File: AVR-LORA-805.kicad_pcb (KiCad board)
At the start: 2 copper layers, 51.7 x 29.2 mm, 39 parts, among them J1 Batt, J2 Solar, J3 SMA, J4 CONN_01X14, J5 CONN_01X14, U1 MCP1700-3302E_SOT23, U2 RFM95HW, U3 AVR128DB28, Y1 24MHz, Y2 32768Hz

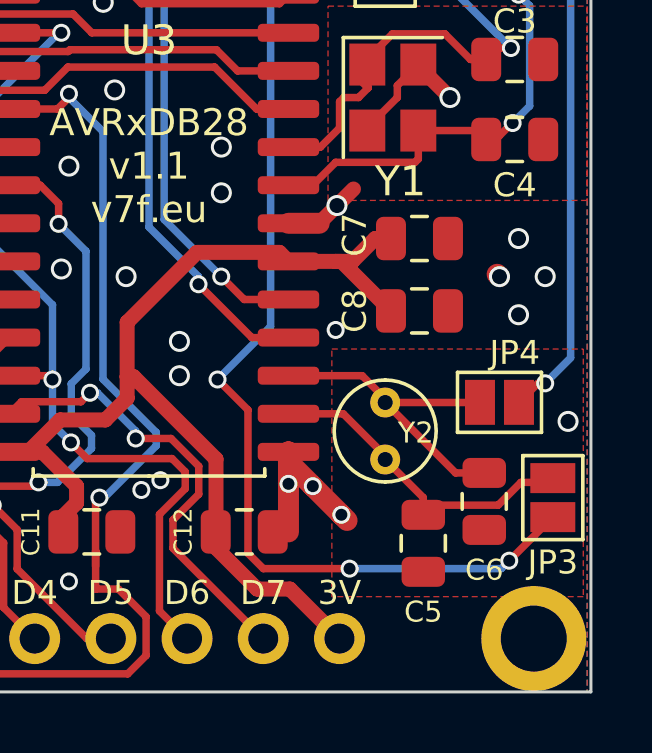
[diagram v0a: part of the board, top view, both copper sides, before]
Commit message: crystal grounding
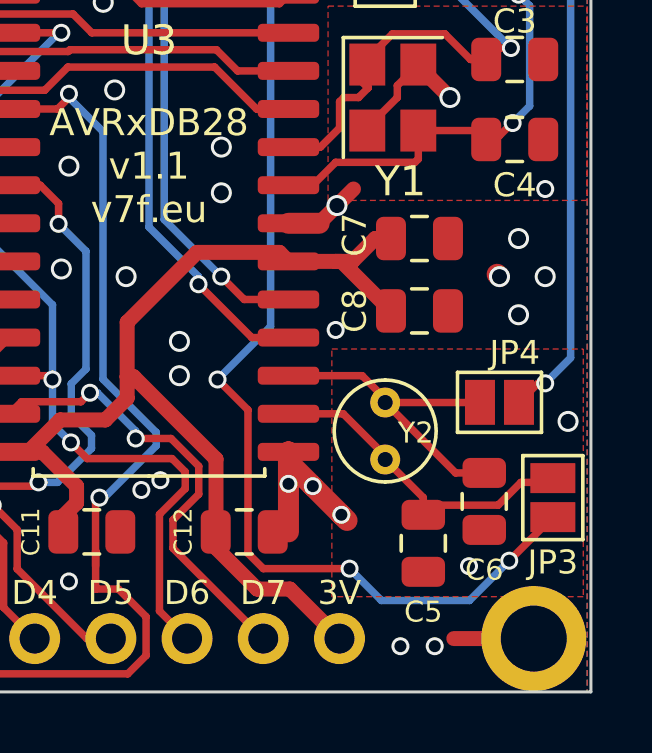
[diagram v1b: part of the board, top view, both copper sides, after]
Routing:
- net GND: track 68.5 -> 71.2 mm, vias 51 -> 55
- net /CF0: track 36.4 -> 37.3 mm
